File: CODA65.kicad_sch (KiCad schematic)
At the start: 32 parts, among them J1 Conn_01x04, J2 Conn_01x05, U1 RP2040, U2 W25Q128JVS, U3 XC6206PxxxMR, Y1 Crystal_GND24

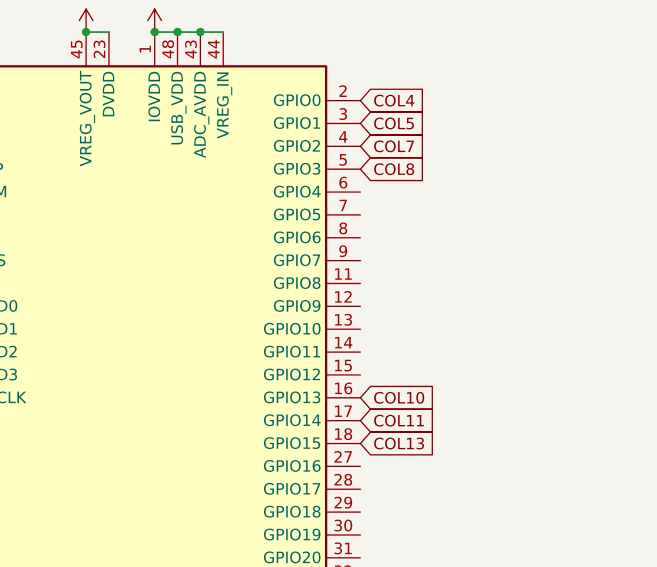
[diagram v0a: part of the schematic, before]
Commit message: Routing Done
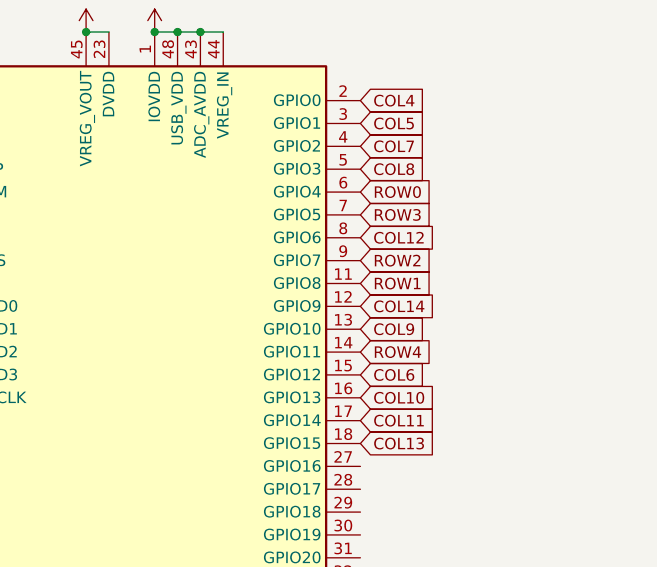
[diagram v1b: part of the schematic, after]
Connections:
- net ROW1: now reaches U1.11 (GPIO8)
- net COL14: now reaches U1.12 (GPIO9)
- net COL9: now reaches U1.13 (GPIO10)
- net ROW4: now reaches U1.14 (GPIO11)
- net COL6: now reaches U1.15 (GPIO12)
- net ROW0: now reaches U1.6 (GPIO4)
- net ROW3: now reaches U1.7 (GPIO5)
- net COL12: now reaches U1.8 (GPIO6)
- net ROW2: now reaches U1.9 (GPIO7)
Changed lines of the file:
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@@
+    )
+  )
+  (global_label "COL12" (shape input) (at 247.65 69.85 0) (fields_autoplaced)
+    (effects (font (size 1.27 1.27)) (justify left))
+    (property "Intersheetrefs" "${INTERSHEET_REFS}" (at 256.6828 69.85 0)
+      (effects (font (size 1.27 1.27)) (justify left) hide)
     )
   )
@@
     )
   )
+  (global_label "ROW1" (shape input) (at 247.65 74.93 0) (fields_autoplaced)
+    (effects (font (size 1.27 1.27)) (justify left))
+    (property "Intersheetrefs" "${INTERSHEET_REFS}" (at 255.8966 74.93 0)
+      (effects (font (size 1.27 1.27)) (justify left) hide)
+    )
+  )
   (global_label "XIN" (shape input) (at 167.64 105.41 0) (fields_autoplaced)
     (effects (font (size 1.27 1.27)) (justify left))
@@
     )
   )
+  (global_label "ROW4" (shape input) (at 247.65 82.55 0) (fields_autoplaced)
+    (effects (font (size 1.27 1.27)) (justify left))
+    (property "Intersheetrefs" "${INTERSHEET_REFS}" (at 255.8966 82.55 0)
+      (effects (font (size 1.27 1.27)) (justify left) hide)
+    )
+  )
   (global_label "RESET" (shape input) (at 196.85 54.61 180) (fields_autoplaced)
     (effects (font (size 1.27 1.27)) (justify right))
@@
     )
   )
+  (global_label "ROW3" (shape input) (at 247.65 67.31 0) (fields_autoplaced)
+    (effects (font (size 1.27 1.27)) (justify left))
+    (property "Intersheetrefs" "${INTERSHEET_REFS}" (at 255.8966 67.31 0)
+      (effects (font (size 1.27 1.27)) (justify left) hide)
+    )
+  )
   (global_label "Q_IO1" (shape input) (at 196.85 80.01 180) (fields_autoplaced)
     (effects (font (size 1.27 1.27)) (justify right))
@@
     )
   )
+  (global_label "COL14" (shape input) (at 247.65 77.47 0) (fields_autoplaced)
+    (effects (font (size 1.27 1.27)) (justify left))
+    (property "Intersheetrefs" "${INTERSHEET_REFS}" (at 256.6828 77.47 0)
+      (effects (font (size 1.27 1.27)) (justify left) hide)
+    )
+  )
   (global_label "XOUT" (shape input) (at 167.64 113.03 0) (fields_autoplaced)
     (effects (font (size 1.27 1.27)) (justify left))
@@
     )
   )
+  (global_label "ROW2" (shape input) (at 247.65 72.39 0) (fields_autoplaced)
+    (effects (font (size 1.27 1.27)) (justify left))
+    (property "Intersheetrefs" "${INTERSHEET_REFS}" (at 255.8966 72.39 0)
+      (effects (font (size 1.27 1.27)) (justify left) hide)
+    )
+  )
   (global_label "Q_IO2" (shape input) (at 196.85 82.55 180) (fields_autoplaced)
     (effects (font (size 1.27 1.27)) (justify right))
@@
     )
   )
+  (global_label "COL6" (shape input) (at 247.65 85.09 0) (fields_autoplaced)
+    (effects (font (size 1.27 1.27)) (justify left))
+    (property "Intersheetrefs" "${INTERSHEET_REFS}" (at 255.4733 85.09 0)
+      (effects (font (size 1.27 1.27)) (justify left) hide)
+    )
+  )
   (global_label "D-" (shape input) (at 182.88 66.04 180) (fields_autoplaced)
     (effects (font (size 1.27 1.27)) (justify right))
@@
     )
   )
+  (global_label "ROW0" (shape input) (at 247.65 64.77 0) (fields_autoplaced)
+    (effects (font (size 1.27 1.27)) (justify left))
+    (property "Intersheetrefs" "${INTERSHEET_REFS}" (at 255.8966 64.77 0)
+      (effects (font (size 1.27 1.27)) (justify left) hide)
+    )
+  )
   (global_label "COL7" (shape input) (at 247.65 59.69 0) (fields_autoplaced)
     (effects (font (size 1.27 1.27)) (justify left))
@@
       (effects (font (size 1.27 1.27)) (justify left) hide)
     )
+  )
+  (global_label "COL9" (shape input) (at 247.65 80.01 0) (fields_autoplaced)
+    (effects (font (size 1.27 1.27)) (justify left))
+    (property "Intersheetrefs" "${INTERSHEET_REFS}" (at 255.4733 80.01 0)
+      (effects (font (size 1.27 1.27)) (justify left) hide)
+    )
